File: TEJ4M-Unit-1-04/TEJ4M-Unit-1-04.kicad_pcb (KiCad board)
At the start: 2 copper layers, 100 x 100 mm, 17 parts, among them J1 XLR3_Switched, J2 XLR3_Switched, J3 Conn_01x02_Socket, Q1 NPN, Q2 NPN, Q3 NPN

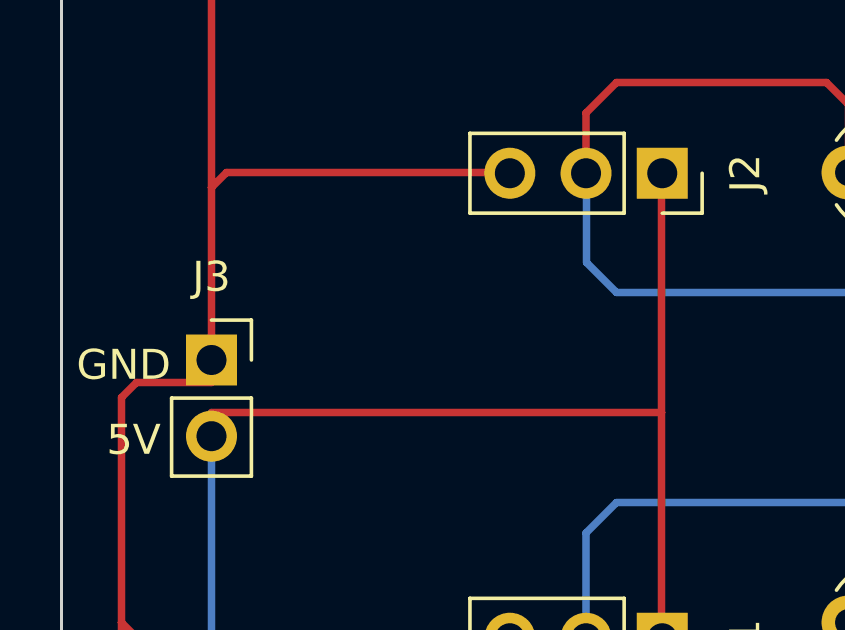
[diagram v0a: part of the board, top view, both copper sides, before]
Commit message: Add files via upload
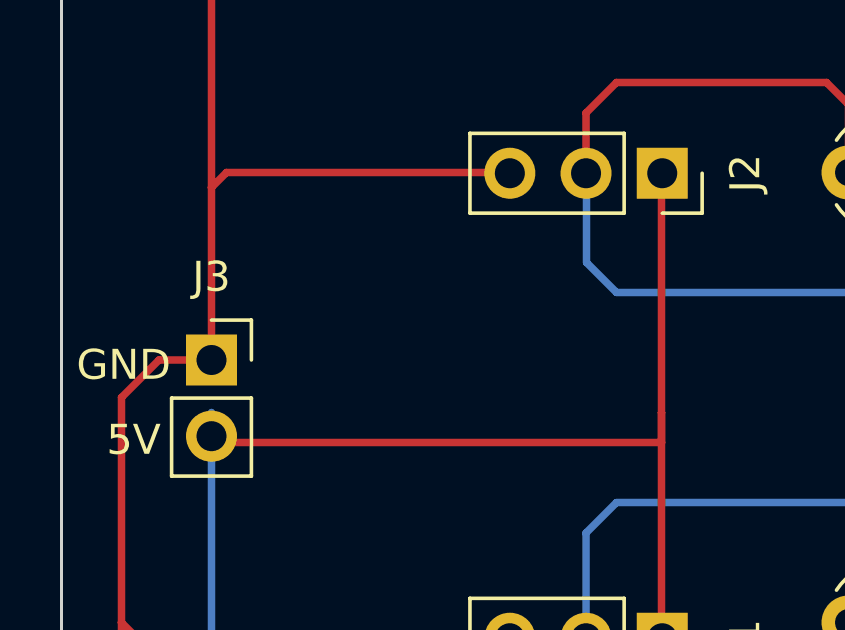
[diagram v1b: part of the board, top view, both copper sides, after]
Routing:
- net Net-(J3-Pin_2): track 148.4 -> 149.5 mm
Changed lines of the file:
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@@
   (segment (start 172.5 80.46) (end 172.5 72.04) (width 0.25) (layer "F.Cu") (net 7))
   (segment (start 120 67.55) (end 120 75.5) (width 0.25) (layer "F.Cu") (net 7))
+  (segment (start 120 76.5) (end 105.21 76.5) (width 0.25) (layer "F.Cu") (net 7))
   (segment (start 120.025 67.525) (end 120 67.55) (width 0.25) (layer "F.Cu") (net 7))
-  (segment (start 120 75.5) (end 105 75.5) (width 0.25) (layer "F.Cu") (net 7))
+  (segment (start 120 75.5) (end 120 76.5) (width 0.25) (layer "F.Cu") (net 7))
   (segment (start 120 83) (end 120 75.5) (width 0.25) (layer "F.Cu") (net 7))
   (segment (start 120.025 83.025) (end 120 83) (width 0.25) (layer "F.Cu") (net 7))
+  (segment (start 105.21 76.5) (end 105 76.29) (width 0.25) (layer "F.Cu") (net 7))
   (segment (start 174.5 97) (end 106 97) (width 0.25) (layer "B.Cu") (net 7))
   (segment (start 173.96 80.46) (end 175.5 82) (width 0.25) (layer "B.Cu") (net 7))
@@
   (segment (start 160.36 86.27) (end 160.36 94.14) (width 0.25) (layer "F.Cu") (net 8))
   (segment (start 125 57.5) (end 106 57.5) (width 0.25) (layer "F.Cu") (net 8))
+  (segment (start 105 73.75) (end 105 68) (width 0.25) (layer "F.Cu") (net 8))
   (segment (start 114.92 67.5) (end 105.5 67.5) (width 0.25) (layer "F.Cu") (net 8))
   (segment (start 106.5 54) (end 105 55.5) (width 0.25) (layer "F.Cu") (net 8))
   (segment (start 160.36 94.14) (end 159.5 95) (width 0.25) (layer "F.Cu") (net 8))
   (segment (start 103 95) (end 102 94) (width 0.25) (layer "F.Cu") (net 8))
+  (segment (start 102 82.5) (end 102 75) (width 0.25) (layer "F.Cu") (net 8))
   (segment (start 114.945 67.525) (end 114.92 67.5) (width 0.25) (layer "F.Cu") (net 8))
   (segment (start 124.96 92.5) (end 104.5 92.5) (width 0.25) (layer "F.Cu") (net 8))
+  (segment (start 103.25 73.75) (end 105 73.75) (width 0.25) (layer "F.Cu") (net 8))
   (segment (start 123.5 54) (end 106.5 54) (width 0.25) (layer "F.Cu") (net 8))
   (segment (start 105.5 67.5) (end 105 68) (width 0.25) (layer "F.Cu") (net 8))
@@
   (segment (start 102 90) (end 102 82.5) (width 0.25) (layer "F.Cu") (net 8))
   (segment (start 104.5 92.5) (end 102 90) (width 0.25) (layer "F.Cu") (net 8))
-  (segment (start 105 68) (end 105 74.5) (width 0.25) (layer "F.Cu") (net 8))
+  (segment (start 102 75) (end 103.25 73.75) (width 0.25) (layer "F.Cu") (net 8))
   (segment (start 105 55.5) (end 105 59) (width 0.25) (layer "F.Cu") (net 8))
   (segment (start 106 57.5) (end 105 58.5) (width 0.25) (layer "F.Cu") (net 8))
   (segment (start 194.04 75) (end 194.04 93.96) (width 0.25) (layer "F.Cu") (net 8))
-  (segment (start 102 75) (end 102.5 74.5) (width 0.25) (layer "F.Cu") (net 8))
   (segment (start 102 94) (end 102 90) (width 0.25) (layer "F.Cu") (net 8))
   (segment (start 194.04 93.96) (end 193 95) (width 0.25) (layer "F.Cu") (net 8))
   (segment (start 159.5 95) (end 103 95) (width 0.25) (layer "F.Cu") (net 8))
-  (segment (start 102.5 74.5) (end 105 74.5) (width 0.25) (layer "F.Cu") (net 8))
-  (segment (start 102 82.5) (end 102 75) (width 0.25) (layer "F.Cu") (net 8))
   (via (at 123.5 54) (size 0.8) (drill 0.4) (layers "F.Cu" "B.Cu") (net 8))
   (segment (start 154.5 67) (end 153 65.5) (width 0.25) (layer "B.Cu") (net 8))
